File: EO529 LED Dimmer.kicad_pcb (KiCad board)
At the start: 2 copper layers, 76.2 x 45.7 mm, 47 parts, among them J1 VBat, Q1 BC639, Q2 BC639, Q3 BC639, Q4 BC639, U1 NE556, U2 NE556

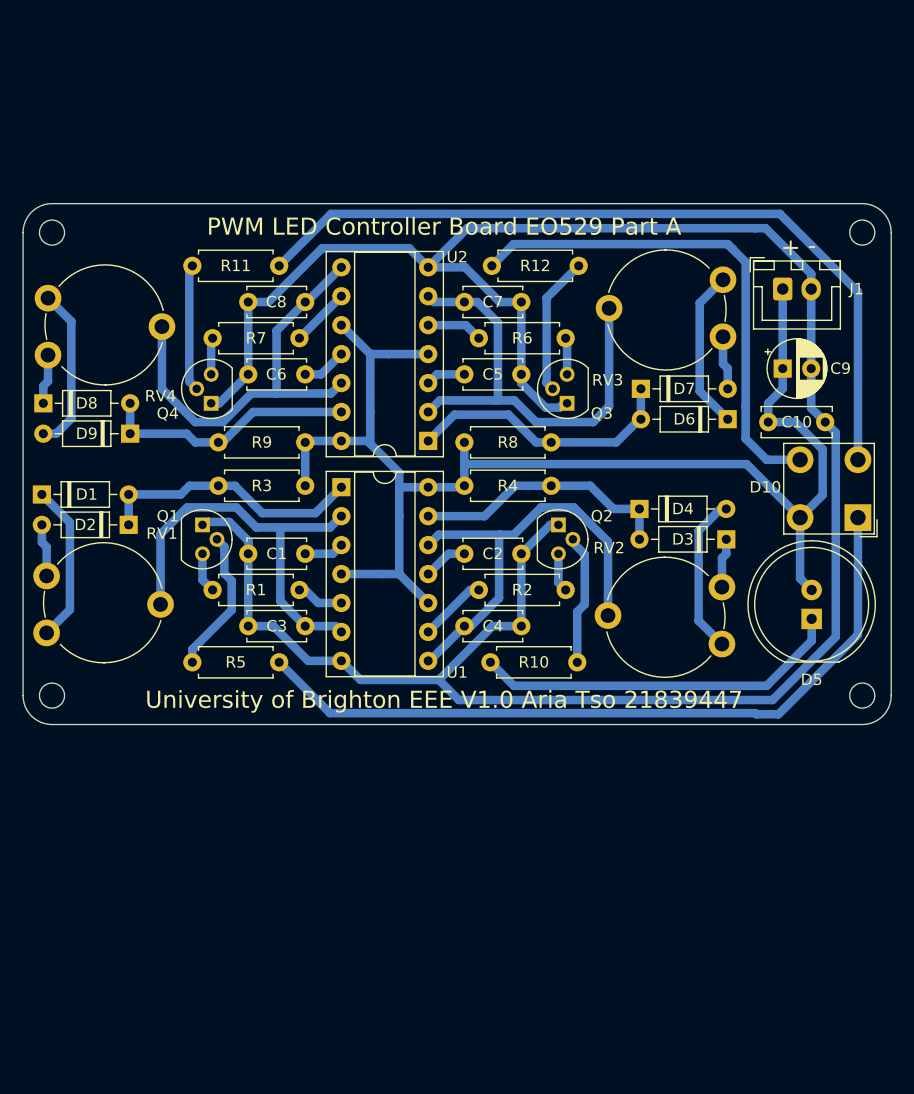
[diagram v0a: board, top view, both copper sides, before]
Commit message: Revision to circuit
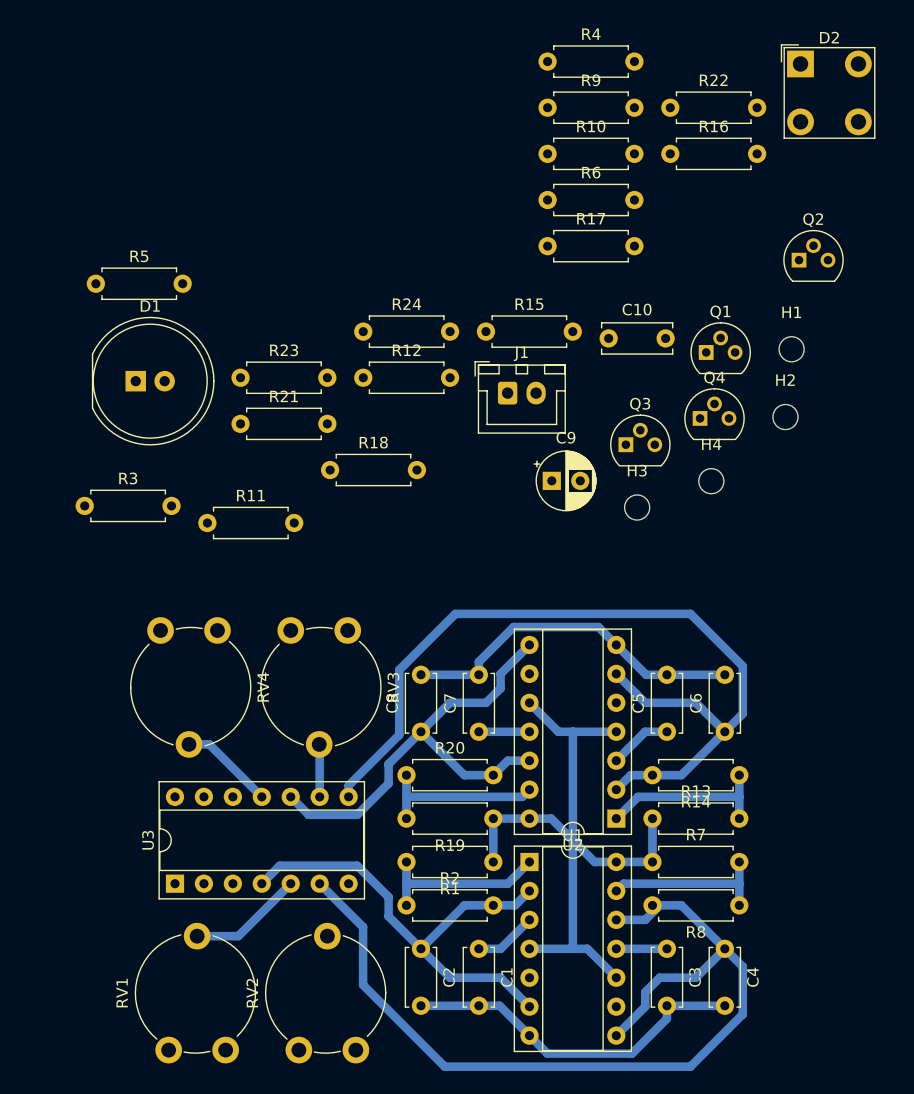
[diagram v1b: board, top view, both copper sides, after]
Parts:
- removed D10: LED_RGBA, LED_THT:LED_BL-FL7680RGB
- removed D3, D4, D6, D7, D8, D9: 1N4148, Diode_THT:D_DO-35_SOD27_P7.62mm_Horizontal
- removed D5: White, LED_THT:LED_D10.0mm
- added R13: 10k, Resistor_THT:R_Axial_DIN0207_L6.3mm_D2.5mm_P7.62mm_Horizontal, F.Cu at (75.3, 81.7)
- added R14: 10k, Resistor_THT:R_Axial_DIN0207_L6.3mm_D2.5mm_P7.62mm_Horizontal, F.Cu at (82.9, 77.9)
- added R15: 100k, Resistor_THT:R_Axial_DIN0207_L6.3mm_D2.5mm_P7.62mm_Horizontal, F.Cu at (60.7, 38.9)
- added R16: 100k, Resistor_THT:R_Axial_DIN0207_L6.3mm_D2.5mm_P7.62mm_Horizontal, F.Cu at (76.9, 23.3)
- added R17: 1k, Resistor_THT:R_Axial_DIN0207_L6.3mm_D2.5mm_P7.62mm_Horizontal, F.Cu at (66.1, 31.4)
- added R18: 180, Resistor_THT:R_Axial_DIN0207_L6.3mm_D2.5mm_P7.62mm_Horizontal, F.Cu at (47.0, 51.1)
- added R19: 10k, Resistor_THT:R_Axial_DIN0207_L6.3mm_D2.5mm_P7.62mm_Horizontal, F.Cu at (61.3, 81.7)
- added R20: 10k, Resistor_THT:R_Axial_DIN0207_L6.3mm_D2.5mm_P7.62mm_Horizontal, F.Cu at (53.7, 77.9)
- added R21: 100k, Resistor_THT:R_Axial_DIN0207_L6.3mm_D2.5mm_P7.62mm_Horizontal, F.Cu at (39.2, 47.0)
- added R22: 100k, Resistor_THT:R_Axial_DIN0207_L6.3mm_D2.5mm_P7.62mm_Horizontal, F.Cu at (76.9, 19.3)
- added R23: 1k, Resistor_THT:R_Axial_DIN0207_L6.3mm_D2.5mm_P7.62mm_Horizontal, F.Cu at (39.2, 43.0)
- added R24: 220, Resistor_THT:R_Axial_DIN0207_L6.3mm_D2.5mm_P7.62mm_Horizontal, F.Cu at (49.9, 38.9)
- added U3: LM339, Package_DIP:DIP-14_W7.62mm_Socket, F.Cu at (33.4, 87.4)
- D1: value 1N4148 -> White; footprint Diode_THT:D_DO-35_SOD27_P7.62mm_Horizontal -> LED_THT:LED_D10.0mm
- D2: value 1N4148 -> LED_RGBA; footprint Diode_THT:D_DO-35_SOD27_P7.62mm_Horizontal -> LED_THT:LED_BL-FL7680RGB
- R1, R2, R7, R8: value 1k -> 10k
- R10, R3, R4, R9: value 1k -> 100k
- R12: value 1k -> 220
- R5: value 180 -> 1k
- R6: value 10k -> 150
- moved D2 71.5 mm to (88.3, 15.4), turned to 0 degrees
- moved H2 68.9 mm to (87.0, 46.4)
- moved H1 65.7 mm to (87.5, 40.5)
- moved R7 60.0 mm to (75.3, 85.5)
- moved RV2 51.8 mm to (49.3, 102.0), turned to 90 degrees
- moved RV3 48.9 mm to (43.6, 65.2), turned to 270 degrees
- moved C6 48.4 mm to (81.7, 74.0), turned to 90 degrees
- moved R8 47.3 mm to (82.9, 89.3), turned to 180 degrees
- moved Q1 46.7 mm to (80.0, 40.7), turned to 0 degrees
- moved R10 44.7 mm to (66.1, 23.3), turned to 0 degrees
- moved Q4 42.9 mm to (79.5, 46.5), turned to 0 degrees
- moved C3 42.5 mm to (76.6, 93.1), turned to 270 degrees
- moved RV1 39.8 mm to (37.8, 102.0), turned to 90 degrees
- moved C8 39.1 mm to (55.0, 74.0), turned to 90 degrees
- moved R4 37.9 mm to (66.1, 15.2)
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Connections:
- D1 pad 2: Net-(D1-Pad2) -> VCC
- D2 pad 1: Net-(D1-Pad2) -> Red
- D2 pad 2: Net-(D2-Pad2) -> Green
- R1 pad 1: Net-(Q1-Pad3) -> VCC
- R10 pad 1: Net-(Q2-Pad2) -> Net-(R10-Pad1)
- R10 pad 2: Net-(D5-Pad1) -> GND
- R11 pad 1: Net-(Q4-Pad2) -> Net-(Q2-Pad3)
- R11 pad 2: Green -> Net-(R11-Pad2)
- R12 pad 1: Net-(Q3-Pad2) -> Net-(Q2-Pad2)
- R12 pad 2: Blue -> Green
- R2 pad 1: Net-(Q2-Pad3) -> Net-(R1-Pad2)
- R2 pad 2: Net-(R2-Pad2) -> Net-(C2-Pad1)
- R3 pad 2: Net-(D1-Pad2) -> Net-(R3-Pad2)
- R4 pad 1: VCC -> Net-(R4-Pad1)
- R4 pad 2: Net-(D3-Pad2) -> GND
- R5 pad 1: Net-(Q1-Pad2) -> Net-(Q1-Pad3)
- R5 pad 2: Red -> Net-(R5-Pad2)
- R6 pad 1: Net-(Q3-Pad3) -> Net-(Q1-Pad2)
- R6 pad 2: Net-(R6-Pad2) -> Red
- R7 pad 1: Net-(Q4-Pad3) -> VCC
- R8 pad 1: VCC -> Net-(R7-Pad2)
- R8 pad 2: Net-(D6-Pad2) -> Net-(C4-Pad1)
- R9 pad 2: Net-(D8-Pad2) -> Net-(R9-Pad2)
- RV1 pad 1: Net-(D1-Pad1) -> Net-(R4-Pad1)
- RV1 pad 2: Net-(C3-Pad1) -> Net-(RV1-Pad2)
- RV1 pad 3: Net-(D2-Pad2) -> Net-(R3-Pad2)
- RV2 pad 1: Net-(D3-Pad1) -> Net-(R10-Pad1)
- RV2 pad 2: Net-(C4-Pad1) -> Net-(RV2-Pad2)
- RV2 pad 3: Net-(D4-Pad2) -> Net-(R9-Pad2)
- RV3 pad 2: Net-(C7-Pad1) -> Net-(RV3-Pad2)
- RV4 pad 2: Net-(C8-Pad1) -> Net-(RV4-Pad2)
- U1 pad 1: Net-(D1-Pad2) -> Net-(R1-Pad2)
- U1 pad 11: Net-(C2-Pad1) -> Net-(C3-Pad1)
- U1 pad 13: Net-(D3-Pad2) -> Net-(R7-Pad2)
- U1 pad 2: Net-(C3-Pad1) -> Net-(C2-Pad1)
- U1 pad 5: Net-(R1-Pad2) -> (no net)
- U1 pad 6: Net-(C3-Pad1) -> Net-(C2-Pad1)
- U1 pad 9: Net-(R2-Pad2) -> (no net)
- U2 pad 1: Net-(D6-Pad2) -> Net-(R13-Pad2)
- U2 pad 11: Net-(C6-Pad1) -> Net-(C7-Pad1)
- U2 pad 13: Net-(D8-Pad2) -> Net-(R19-Pad2)
- U2 pad 2: Net-(C7-Pad1) -> Net-(C6-Pad1)
- U2 pad 5: Net-(R6-Pad2) -> (no net)
- U2 pad 6: Net-(C7-Pad1) -> Net-(C6-Pad1)
- U2 pad 9: Net-(R7-Pad2) -> (no net)
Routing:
- net GND: track 210.0 -> 61.6 mm
- net Net-(C6-Pad1): track 3.91 -> 76.7 mm
- net Green: track 70.3 -> 0.00 mm
- net Red: track 65.9 -> 0.00 mm
- net VCC: track 119.5 -> 59.6 mm
- net Blue: track 44.4 -> 0.00 mm
- net Net-(C4-Pad1): track 39.2 -> 80.8 mm
- net Net-(C2-Pad1): track 3.91 -> 41.9 mm
- net Net-(C7-Pad1): track 40.2 -> 4.45 mm
- net Net-(C3-Pad1): track 37.2 -> 4.45 mm
- net Net-(D5-Pad1): track 32.6 -> 0.00 mm
- net Net-(D6-Pad2): track 24.0 -> 0.00 mm
- net Net-(D1-Pad2): track 23.6 -> 0.00 mm
- net Net-(D3-Pad2): track 23.2 -> 0.00 mm
- net Net-(D8-Pad2): track 22.6 -> 0.00 mm
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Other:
- board outline removed
- board text removed: "+ -"
- board text removed: "PWM LED Controller Board EO529 Part A"
- board text removed: "University of Brighton EEE V1.0 Aria Tso 21839447"
